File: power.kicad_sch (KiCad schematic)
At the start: 31 parts, among them Q4001 DMG1012T-7, U4001 AP62301_TSOT, U4002 TLV76701_WSON

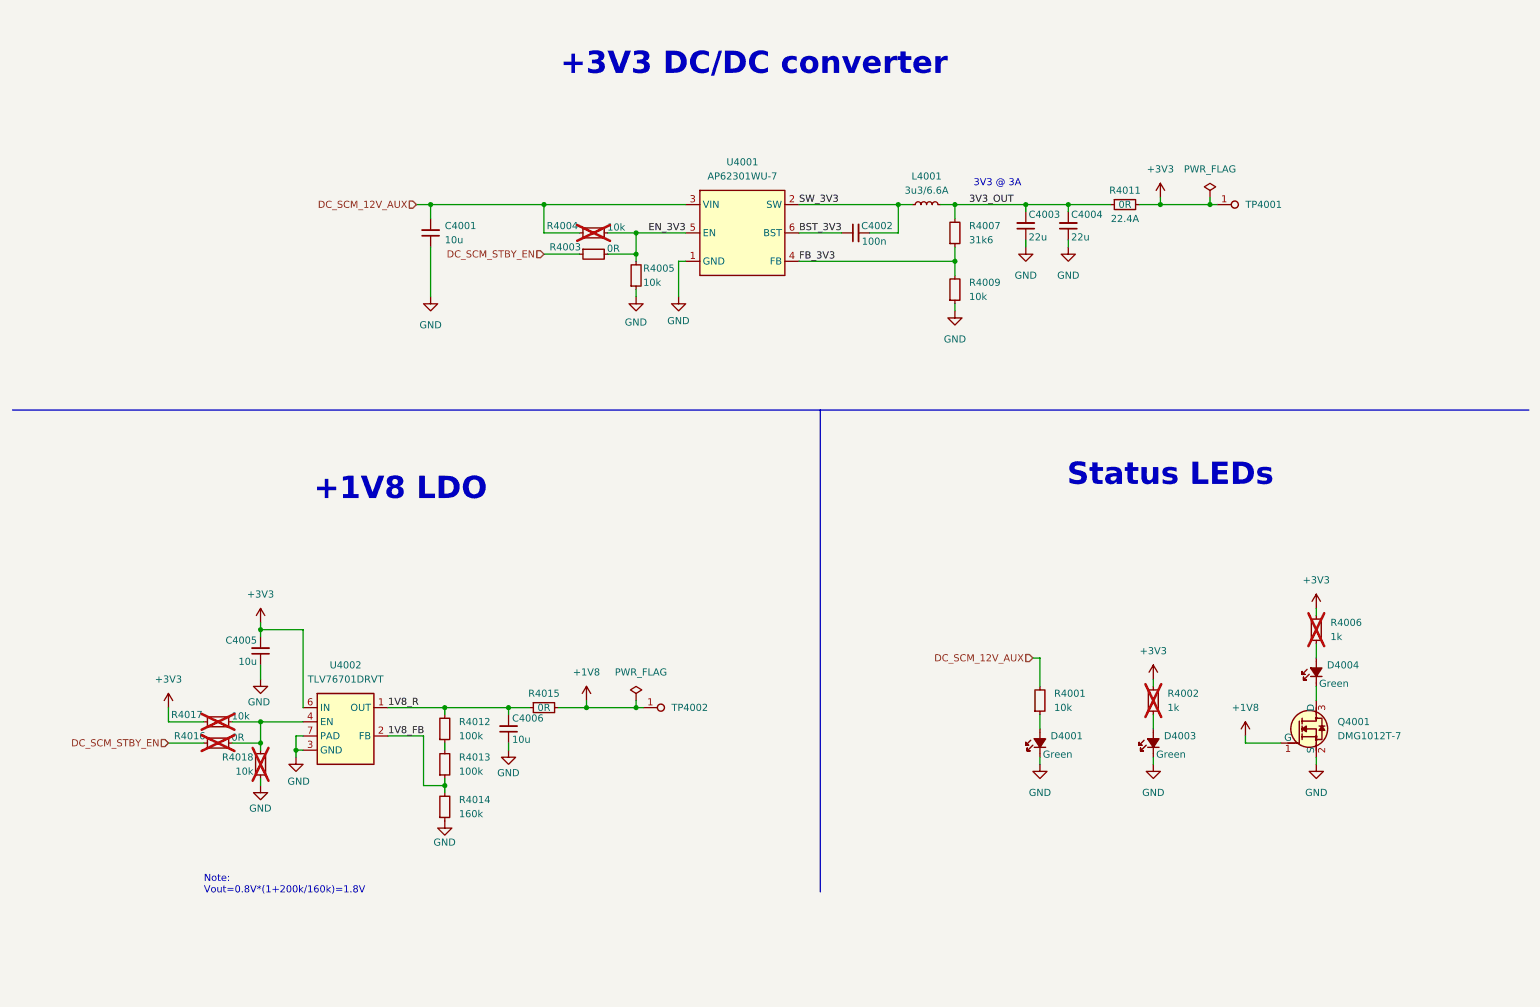
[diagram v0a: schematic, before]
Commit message: [#103910] Update power section
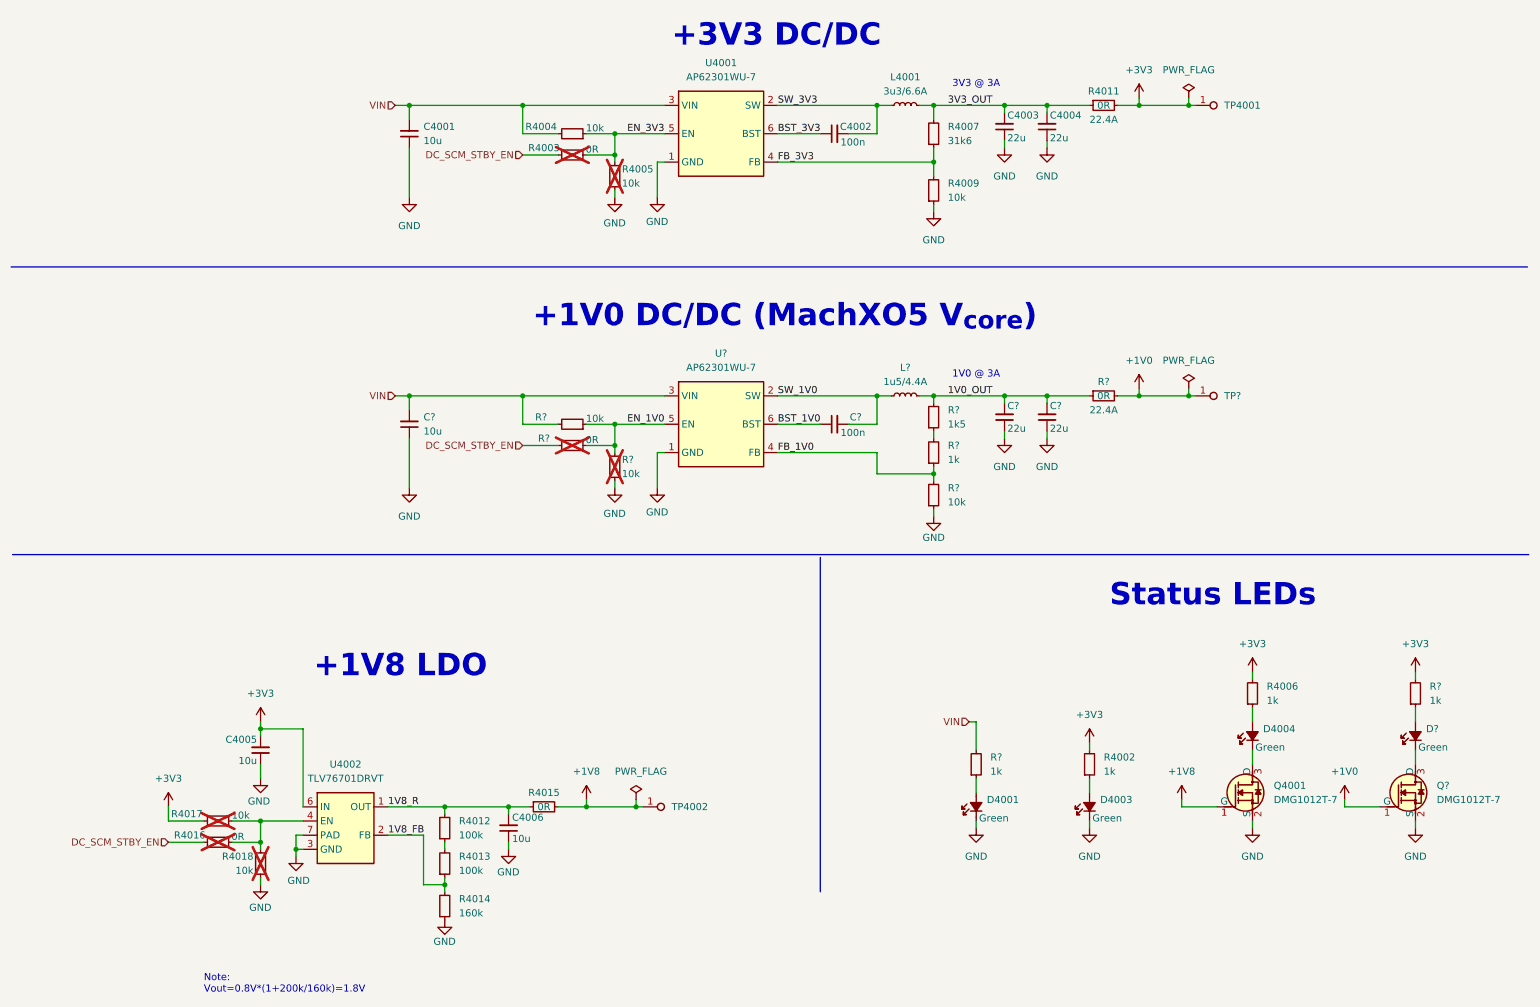
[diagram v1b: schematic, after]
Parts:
- removed R4001: R_10k_0402, antmicro-footprints:R_0402_1005Metric, symbol antmicroResistors0402:R_10k_0402
- added C?: C_22u_16V_0603, antmicro-footprints:C_0603_1608Metric_EIA, symbol antmicroCapacitors0603:C_22u_16V_0603
- added C?: C_22u_0603, antmicro-footprints:C_0603_1608Metric, symbol antmicroCapacitors0603:C_22u_0603
- added C?: C_100n_50V_X8L_0402, antmicro-footprints:C_0402_1005Metric, symbol antmicroCapacitors0402:C_100n_50V_X8L_0402
- added C?: C_10u_16V_0603, antmicro-footprints:C_0603_1608Metric, symbol antmicroCapacitors0603:C_10u_16V_0603
- added D?: LED_G_0603_LTST-C190GKT, antmicro-footprints:LED_0603_1608Metric_G, symbol antmicroLEDIndicationDiscrete:LED_G_0603_LTST-C190GKT
- added L?: L_1u5_4.4A_Bourns-SRP3212A, antmicro-footprints:L_Bourns-SRP3212A, symbol antmicroFixedInductors:L_1u5_4.4A_Bourns-SRP3212A
- added Q?: DMG1012T-7, antmicro-footprints:SOT-523, symbol antmicroTransistorsFETsMOSFETsSingle:DMG1012T-7
- added R? (x3): R_10k_0402, antmicro-footprints:R_0402_1005Metric, symbol antmicroResistors0402:R_10k_0402
- added R? (x3): R_1k_0402, antmicro-footprints:R_0402_1005Metric, symbol antmicroResistors0402:R_1k_0402
- added R?: R_0R_0402, antmicro-footprints:R_0402_1005Metric, symbol antmicroResistors0402:R_0R_0402
- added R?: R_0R_22.4A_0603, antmicro-footprints:R_0603_1608Metric, symbol antmicroResistors0603:R_0R_22.4A_0603
- added R?: R_1k5_0402, antmicro-footprints:R_0402_1005Metric, symbol antmicroResistors0402:R_1k5_0402
- added TP?: TP_0.75mm_SMD, antmicro-footprints:TP_SMD_0.75mm, symbol antmicroTestPoints:TP_0.75mm_SMD
- added U?: AP62301_TSOT, antmicro-footprints:TSOT23-6, symbol antmicroDCDCConverters:AP62301_TSOT
- R4002, R4004, R4006: now fitted
- R4003, R4005: now not fitted; now in the parts list
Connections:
- net +3V3: now also R?.2
- net DC_SCM_STBY_EN: now also R?.1
- net GND: now also C?.1, C?.1, C?.1, Q?.2 (S), R?.1, R?.1, U?.1 (GND)
- net at D4001.2 (A): now also R?.1
- net DC_SCM_12V_AUX renamed VIN
- net VIN: now also C?.2, R?.2, R?.2, U?.3 (VIN)
- new net: D?.1 (C), Q?.3 (D)
- new net: D?.2 (A), R?.1
- new net: R?.1, R?.2
- new net +1V0: Q?.1 (G), R?.2, TP?.1
- new net 1V0_OUT: C?.2, C?.2, L?.2, R?.1, R?.2
- new net BST_1V0: C?.1, U?.6 (BST)
- new net EN_1V0: R?.1, R?.2, R?.2, U?.5 (EN)
- new net FB_1V0: R?.1, R?.2, U?.4 (FB)
- new net SW_1V0: C?.2, L?.1, U?.2 (SW)
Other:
- note added: "+1V0 DC/DC (MachXO5 V_{core})"
- note added: "+3V3 DC/DC"
- note added: "1V0 @ 3A"
- note removed: "+3V3 DC/DC converter"
- moved on the sheet: C4001, C4002, C4003, C4004, C4005, C4006, D4001, D4003, D4004, L4001, Q4001, R4007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
